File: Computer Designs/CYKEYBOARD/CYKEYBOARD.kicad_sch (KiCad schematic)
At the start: 407 parts, among them J1 Conn_01x12, J2 Conn_01x03, J3 Conn_01x03, K0 RESET, K1 F1, K10 F10, K11 F11, K12 F12, K13 READY, K14 ~~,,,,,,`, K15 !,,,,,,1, K16 @,,,,,,2, K17 #,,,,,,3, K18 $,,,,,,4, K19 %,,,,,,5, K2 F2, K20 ^,,,,,,6, K21 &,,,,,,7, K22 *,,,,,,8, K23 (,,,,,,9, K24 ),,,,,,0, K25 _,,,,,,-, K26 +,,,,,,=, K27 BACKSPACE, K28 INS, K29 HOME, K3 F3, K30 !,,,,,,1, K31 SAVE,,,,,,LOAD, K32 Q, K33 W, K34 E, K35 R, K36 T, K37 Y, K38 U, K39 I, K4 F4, K40 O, K41 P, K42 {,,,,,,[, K43 },,,,,,], K44 |,,,,,,\, K45 DEL, K46 HOLD, K47 @,,,,,,2, K48 SHIFT,,,,,,LOCK, K49 A, K5 F5, K50 S, K51 D, K52 F, K53 G, K54 H, K55 J, K56 K, K57 L, K58 :,,,,,,;, K59 ",,,,,,', K6 F6, K60 ENTER, K61 SHIFT, K62 Z, K63 X, K64 C, K65 V, K66 B, K67 N, K68 M, K69 <,,,,,,,, K7 F7, K70 >,,,,,,., K71 ?,,,,,,/, K72 SHIFT, K73 ^, K74 CTRL, K75 CYKA,,,,,,TECH, K76 ALT, K77 Blank, K78 ALT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

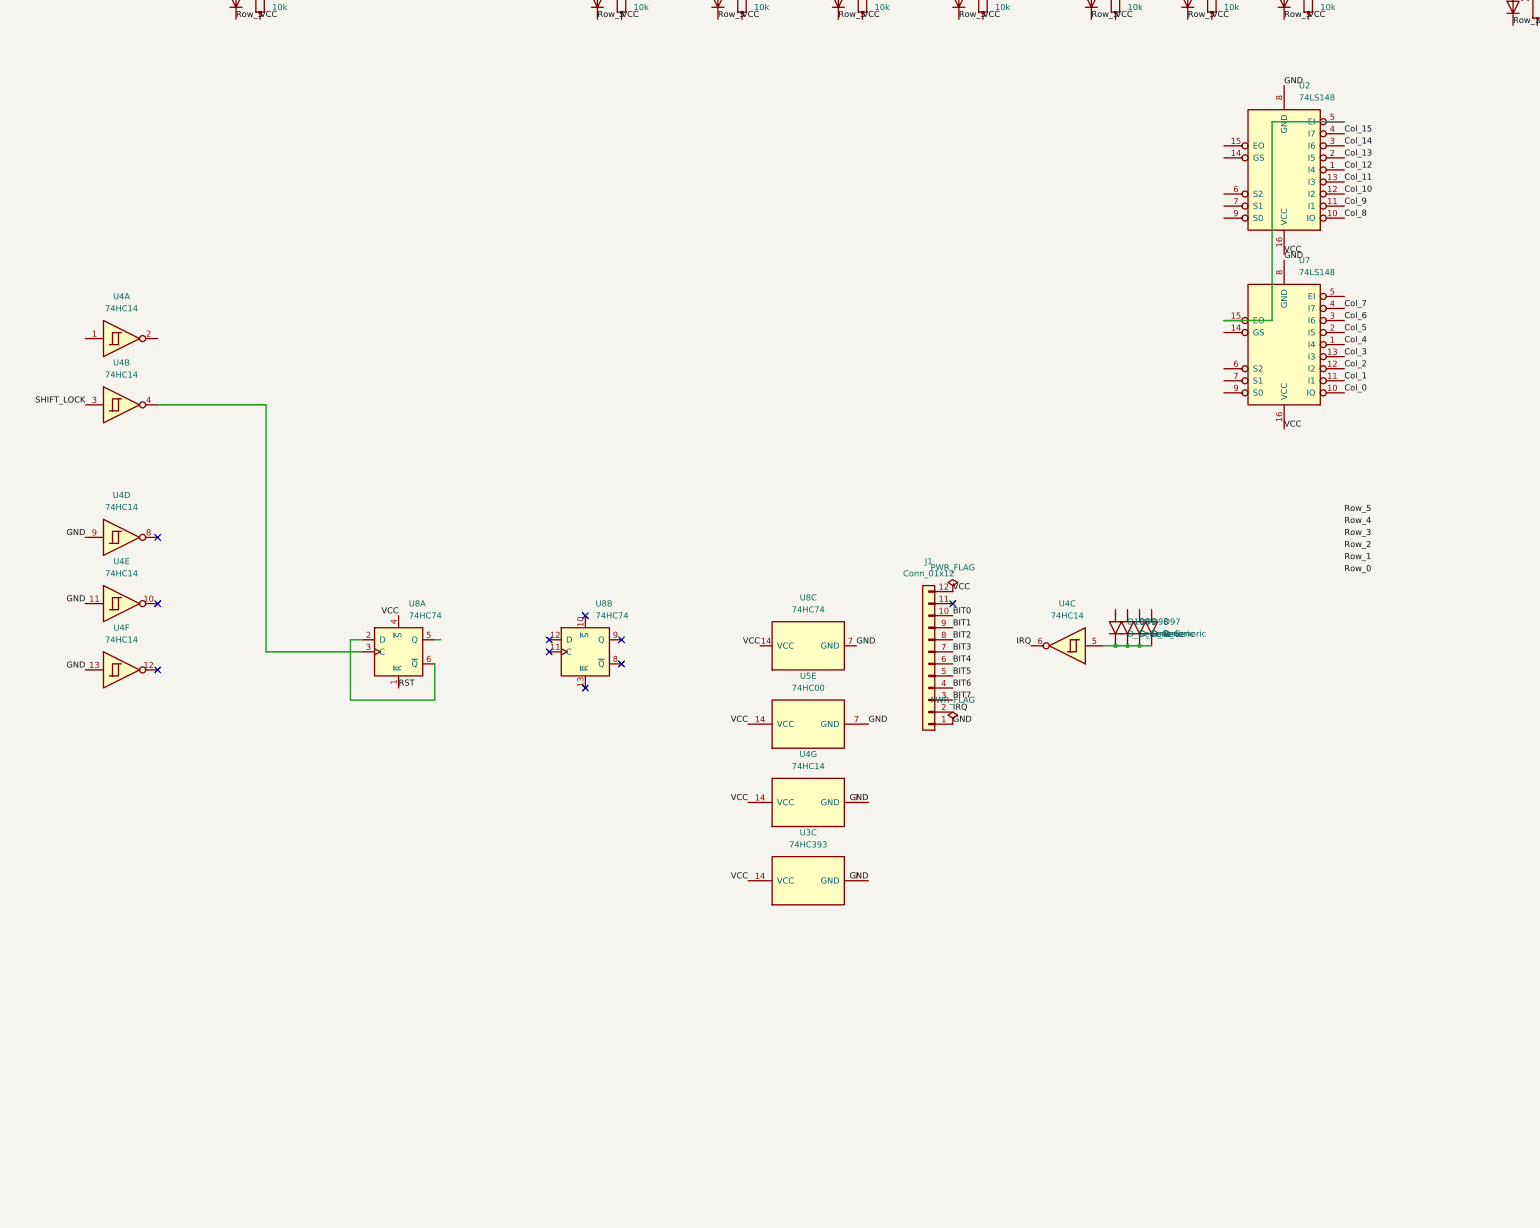
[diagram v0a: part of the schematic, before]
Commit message: changes
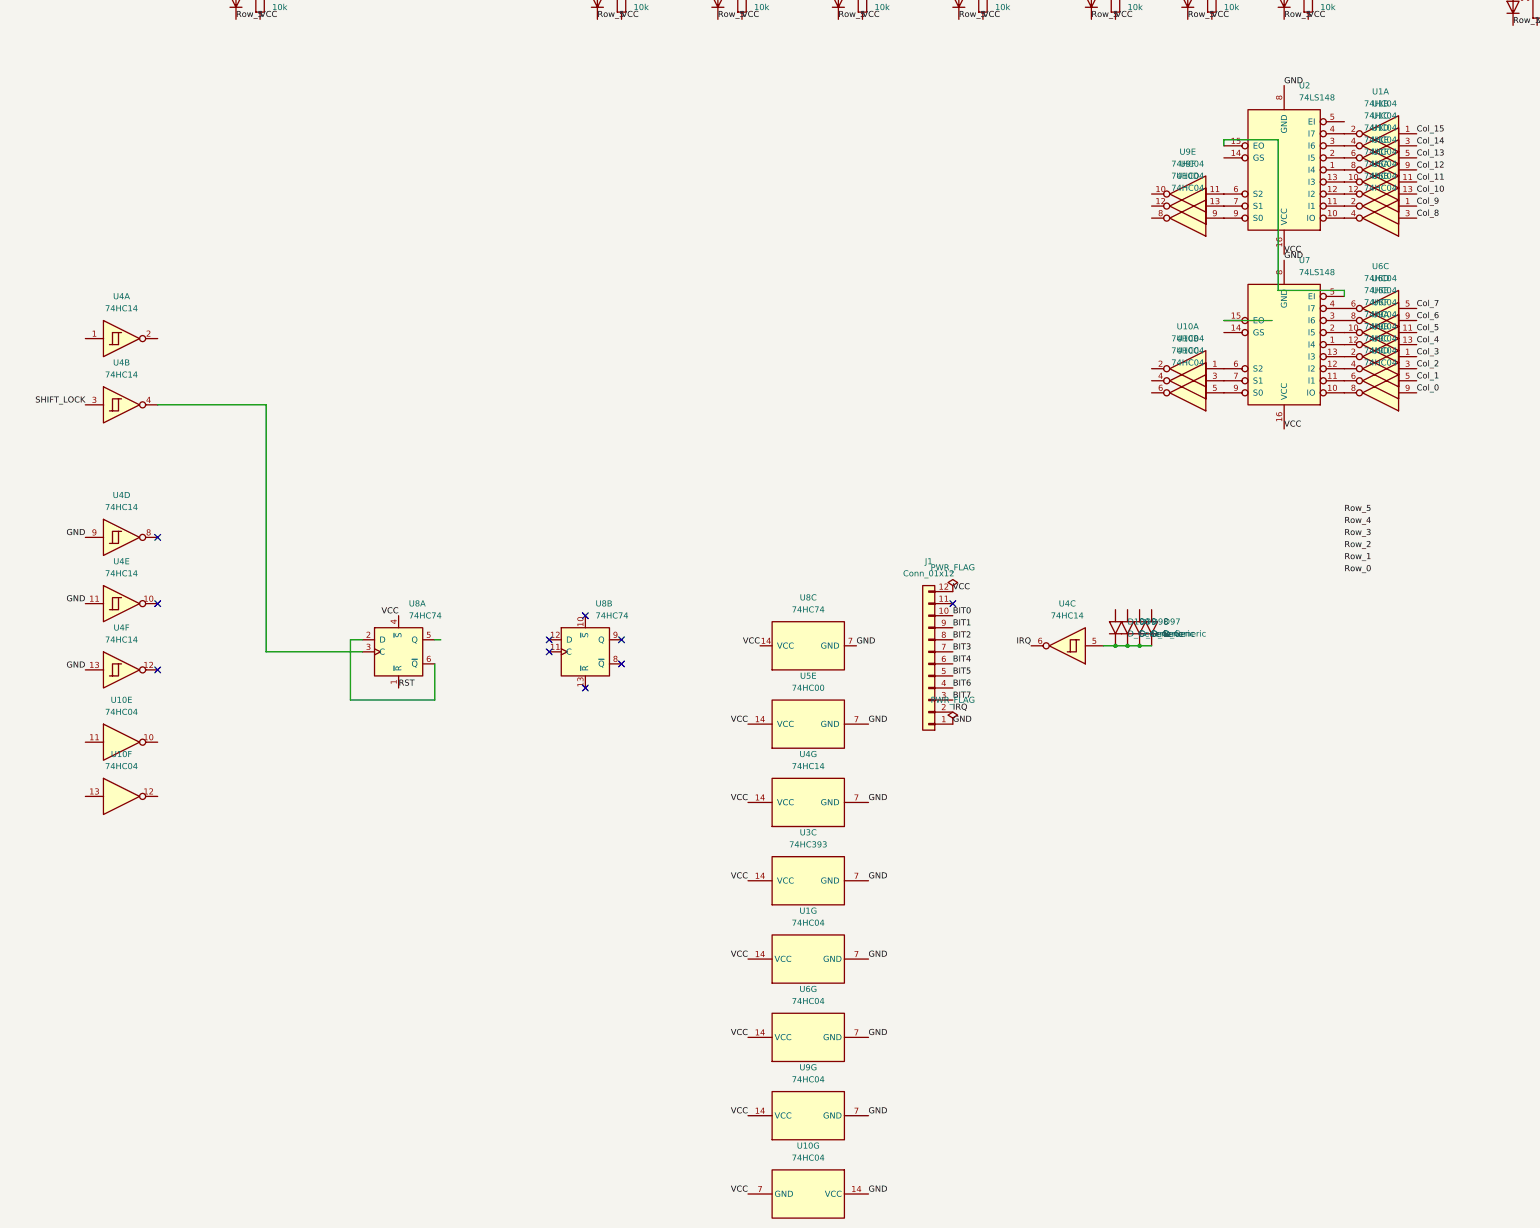
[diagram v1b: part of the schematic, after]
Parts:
- added U1, U10, U6, U9: 74HC04, symbol 74xx:74HC04
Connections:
- net Col_0: now also U9.9; no longer U7.10 (IO)
- net Col_1: now also U9.5; no longer U7.11 (I1)
- net Col_10: now also U1.13; no longer U2.12 (I2)
- net Col_11: now also U1.11; no longer U2.13 (I3)
- net Col_12: now also U1.9; no longer U2.1 (I4)
- net Col_13: now also U1.5; no longer U2.2 (I5)
- net Col_14: now also U1.3; no longer U2.3 (I6)
- net Col_15: now also U1.1; no longer U2.4 (I7)
- net Col_2: now also U9.3; no longer U7.12 (I2)
- net Col_3: now also U9.1; no longer U7.13 (I3)
- net Col_4: now also U6.13; no longer U7.1 (I4)
- net Col_5: now also U6.11; no longer U7.2 (I5)
- net Col_6: now also U6.9; no longer U7.3 (I6)
- net Col_7: now also U6.5; no longer U7.4 (I7)
- net Col_8: now also U6.3; no longer U2.10 (IO)
- net Col_9: now also U6.1; no longer U2.11 (I1)
- net GND: now also U1.7 (GND), U10.14 (VCC), U6.7 (GND), U9.7 (GND)
- net VCC: now also U1.14 (VCC), U10.7 (GND), U6.14 (VCC), U9.14 (VCC)
- net at U7.15 (EO): no longer U2.5 (EI)
- net at U7.5 (EI): now also U2.15 (EO)
- net at U7.6 (S2): now also U10.1
- net at U7.7 (S1): now also U10.3
- net at U7.9 (S0): now also U10.5
- net at U2.6 (S2): now also U9.11
- net at U2.7 (S1): now also U9.13
- net at U2.9 (S0): now also U10.9
- new net: U1.8, U2.1 (I4)
- new net: U2.10 (IO), U6.4
- new net: U6.10, U7.2 (I5)
- new net: U1.6, U2.2 (I5)
- new net: U6.12, U7.1 (I4)
- new net: U7.13 (I3), U9.2
- new net: U6.6, U7.4 (I7)
- new net: U7.11 (I1), U9.6
- new net: U1.10, U2.13 (I3)
- new net: U1.12, U2.12 (I2)
- new net: U6.8, U7.3 (I6)
- new net: U1.4, U2.3 (I6)
- new net: U7.10 (IO), U9.8
- new net: U7.12 (I2), U9.4
- new net: U2.11 (I1), U6.2
- new net: U1.2, U2.4 (I7)
